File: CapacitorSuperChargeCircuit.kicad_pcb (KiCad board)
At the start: 2 copper layers, 49.9 x 15.4 mm, 19 parts, among them J2 Screw_Terminal_01x02, J3 Screw_Terminal_01x02, U1 PAM2421AECADJR

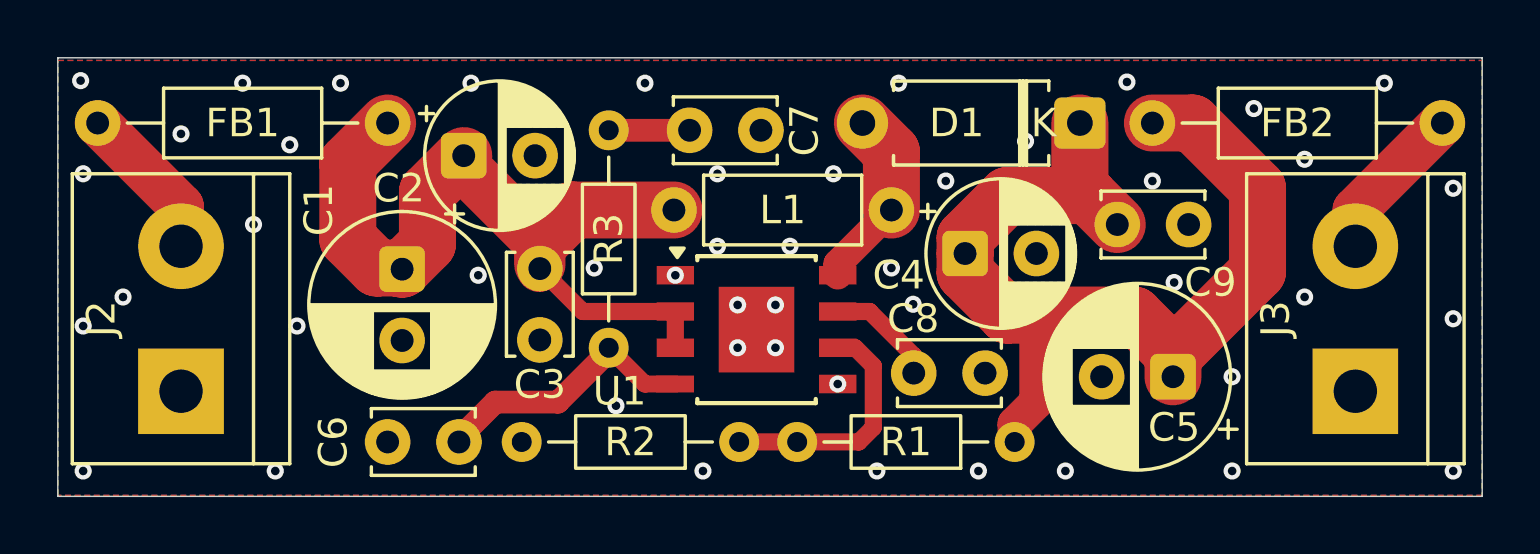
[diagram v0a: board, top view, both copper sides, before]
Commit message: v2 smd version foxed
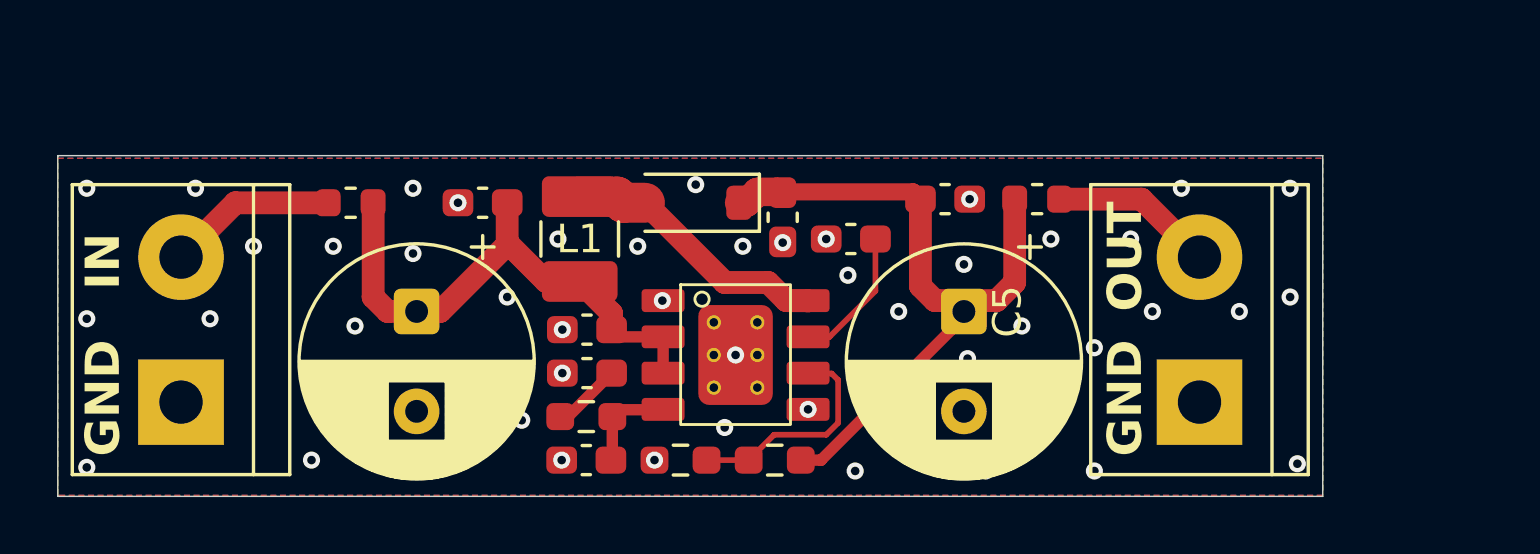
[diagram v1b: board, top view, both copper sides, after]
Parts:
- C1, C5: value 470uF -> 16V 470uF; footprint Capacitor_THT:CP_Radial_D6.3mm_P2.50mm -> Capacitor_THT:CP_Radial_D8.0mm_P3.50mm
- C2, C4: value 10uF -> 10μF 16V X5R; footprint Capacitor_THT:CP_Radial_D5.0mm_P2.50mm -> Capacitor_SMD:C_0603_1608Metric_Pad1.08x0.95mm_HandSolder
- C3, C9: value 1uF -> 1μF 25V X7R; footprint Capacitor_THT:C_Disc_D3.4mm_W2.1mm_P2.50mm -> Capacitor_SMD:C_0603_1608Metric_Pad1.08x0.95mm_HandSolder
- C6: value 47pF -> 47pF 50V CH; footprint Capacitor_THT:C_Disc_D3.4mm_W2.1mm_P2.50mm -> Capacitor_SMD:C_0603_1608Metric_Pad1.08x0.95mm_HandSolder
- C7: value 2.2nF -> 2.2nF 50V X7R; footprint Capacitor_THT:C_Disc_D3.4mm_W2.1mm_P2.50mm -> Capacitor_SMD:C_0603_1608Metric_Pad1.08x0.95mm_HandSolder
- C8: value 10nF -> 0.1μF 50V X7R; footprint Capacitor_THT:C_Disc_D3.4mm_W2.1mm_P2.50mm -> Capacitor_SMD:C_0603_1608Metric_Pad1.08x0.95mm_HandSolder
- D1: value D_Schottky -> RB160M-30TR; footprint Diode_THT:D_A-405_P7.62mm_Horizontal -> Diode_SMD:D_SOD-123
- FB1, FB2: value FerriteBead -> BLM18PG471SN1D; footprint Inductor_THT:L_Axial_L5.3mm_D2.2mm_P10.16mm_Horizontal_Vishay_IM-1 -> Inductor_SMD:L_0603_1608Metric
- L1: value 6.8uH -> DFE322512F-100M; footprint Inductor_THT:L_Axial_L5.3mm_D2.2mm_P7.62mm_Horizontal_Vishay_IM-1 -> Inductor_SMD:L_1210_3225Metric_Pad1.42x2.65mm_HandSolder
- R1: value 85k -> 110k; footprint Resistor_THT:R_Axial_DIN0204_L3.6mm_D1.6mm_P7.62mm_Horizontal -> Resistor_SMD:R_0603_1608Metric_Pad0.98x0.95mm_HandSolder
- R2: value 10k -> 13k; footprint Resistor_THT:R_Axial_DIN0204_L3.6mm_D1.6mm_P7.62mm_Horizontal -> Resistor_SMD:R_0603_1608Metric_Pad0.98x0.95mm_HandSolder
- R3: footprint Resistor_THT:R_Axial_DIN0204_L3.6mm_D1.6mm_P7.62mm_Horizontal -> Resistor_SMD:R_0603_1608Metric_Pad0.98x0.95mm_HandSolder
- U1: value PAM2421AECADJR -> ~; footprint Package_SO:Infineon_PG-DSO-8-43 -> Library:PAM242x
- moved D1 13.9 mm to (167.8, 81.3)
- moved C9 11.7 mm to (170.9, 81.8), turned to -90 degrees
- moved C7 9.24 mm to (164.1, 87.2), turned to 180 degrees
- moved R1 8.43 mm to (170.7, 90.3)
- moved C5 7.67 mm to (177.3, 85.1), turned to -90 degrees
- moved J3 5.47 mm to (185.5, 88.3)
- moved U1 5.38 mm to (169.3, 91.1)
- moved C8 5.19 mm to (173.3, 82.5), turned to 180 degrees
- moved FB2 4.84 mm to (179.9, 81.2)
- moved C6 4.51 mm to (164.1, 90.3)
- moved L1 3.45 mm to (163.8, 82.5), turned to 90 degrees
- moved FB1 3.08 mm to (155.8, 81.3)
- moved C3 2.70 mm to (164.1, 85.7), turned to 180 degrees
- moved R3 2.54 mm to (164.1, 88.8), turned to 180 degrees
- moved R2 2.15 mm to (167.4, 90.3)
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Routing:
- net VOUT: track 37.4 -> 24.5 mm
- net VIN: track 28.8 -> 19.1 mm
- net COMP: track 9.62 -> 3.42 mm
- net SW: track 6.53 -> 9.53 mm
- net FB: track 8.86 -> 7.80 mm
- net SS: track 3.92 -> 4.85 mm
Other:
- board size 49.9 x 15.4 mm -> 44.3 x 11.9 mm
- board text added: "GND"
- board text added: "IN"
- board text added: "OUT"
- board text removed: "CapacitorSuperChargeCircuit"
